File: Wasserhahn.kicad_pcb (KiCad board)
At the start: 2 copper layers, 90.2 x 77.5 mm, 18 parts, among them J1 Mains, J2 Ball_Valve_Contacts, J3 ToRelais, J4 PRGM_ADAPTER, J5 Boot/PRGM, U1 ESP-WROOM-02

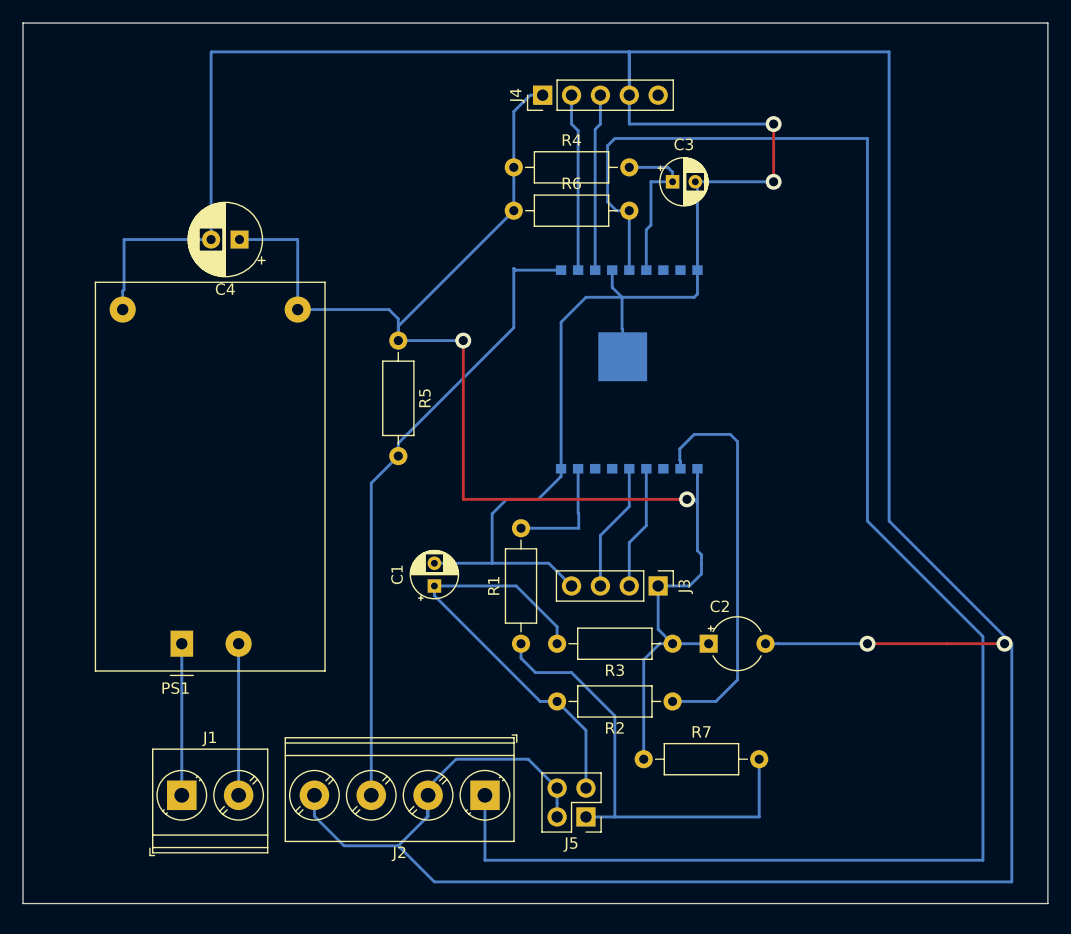
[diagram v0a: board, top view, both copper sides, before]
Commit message: Updated Board and Plot data
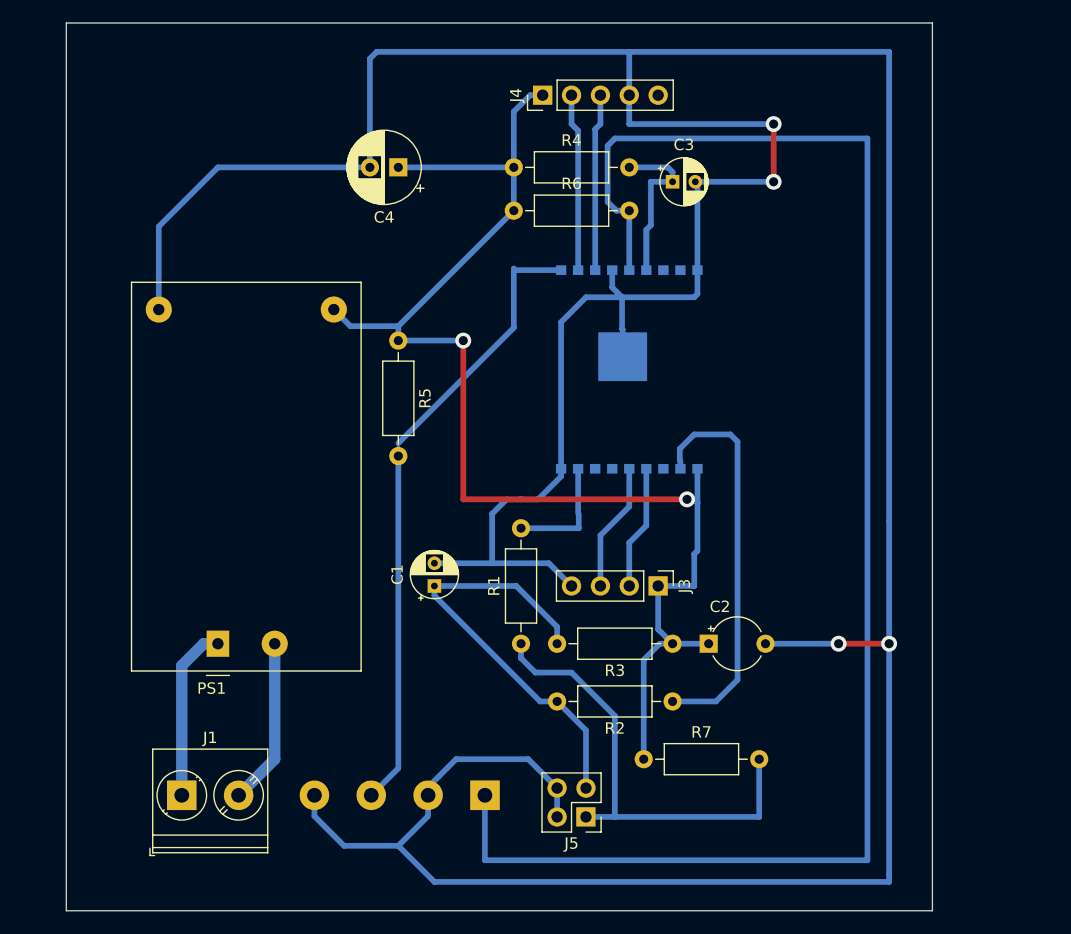
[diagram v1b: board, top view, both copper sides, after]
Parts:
- J2: moved to B.Cu
- moved C4 15.3 mm to (139.7, 40.6)
- moved PS1 3.17 mm to (123.8, 82.5)
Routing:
- net /GND: track 383.6 -> 353.0 mm
- net /Input_Open: track 152.8 -> 138.4 mm
- net /VCC3V3: track 124.6 -> 118.6 mm
- net Net-(J1-Pad1): track 13.3 -> 15.4 mm
- net Net-(J1-Pad2): track 13.3 -> 14.7 mm
- net /Input_Close: track 55.8 -> 56.8 mm
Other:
- board size 90.2 x 77.5 mm -> 76.2 x 78.1 mm
